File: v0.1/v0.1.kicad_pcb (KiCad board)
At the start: 4 copper layers, 66.4 x 47.2 mm, 147 parts, among them J1 Conn_01x05_Pin, J2 Conn_01x04_Pin, J3 Conn_01x02_Pin, J4 Conn_01x02_Pin, U1 XC6206P152MR, U10 STM32U5G9ZJTxQ, U2 XC6206P282MR, U3 SY8088AAC, U4 XC6206P282MR, U9 MX66LM1G45G, X1 32.768kHz, X2 16MHz

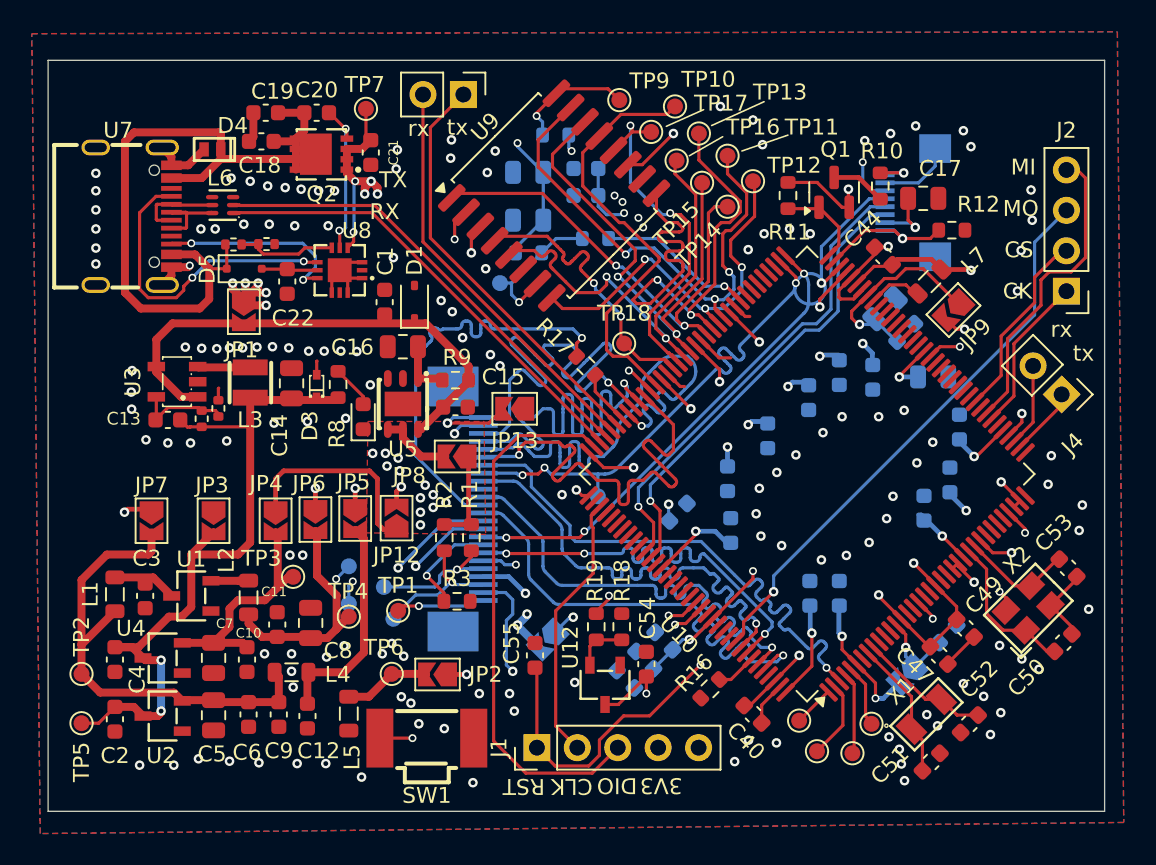
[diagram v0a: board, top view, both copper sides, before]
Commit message: [HW] [PCB] PCB Revision 0.2_Y50; DK1
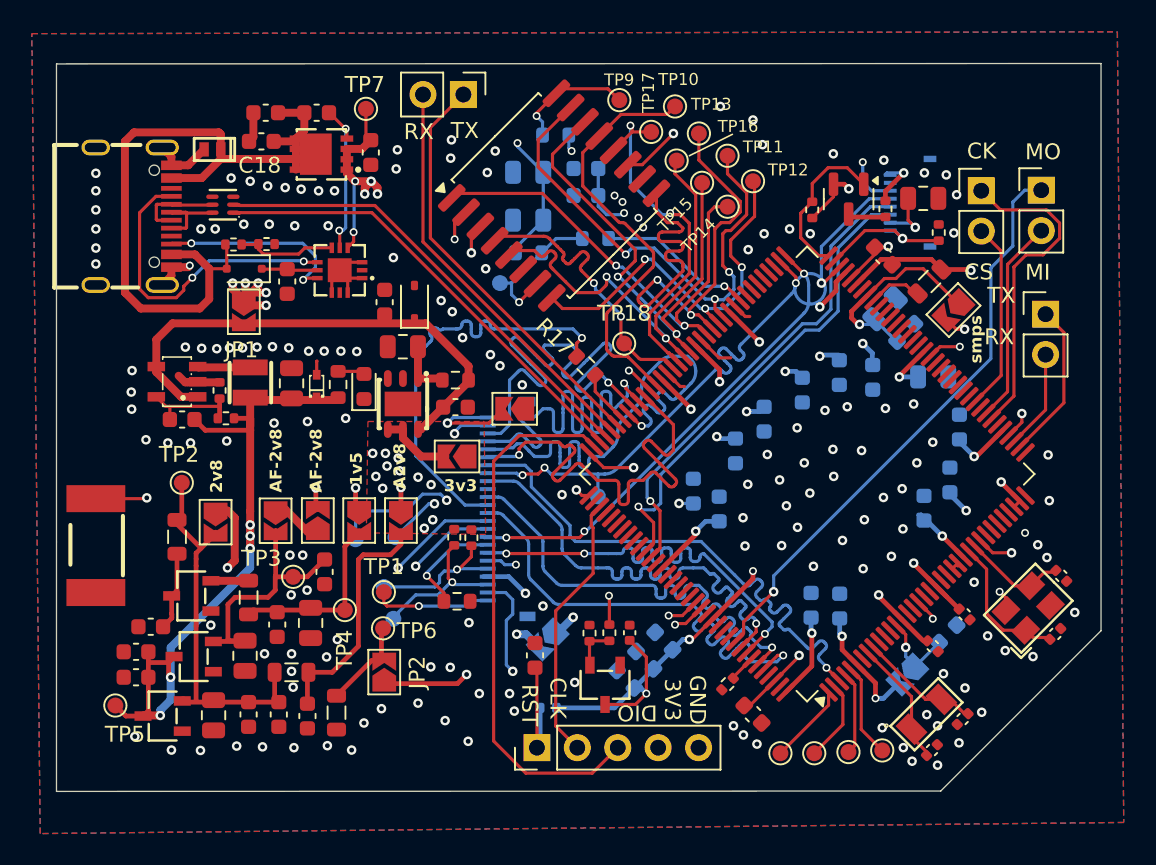
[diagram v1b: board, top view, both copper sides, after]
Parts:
- removed the JP3 at (93.9, 76.5)
- added J3: Conn_01x02_Pin, Connector_PinHeader_2.54mm:PinHeader_1x02_P2.54mm_Vertical, F.Cu at (142.2, 55.8)
- added R20: 100k, Resistor_SMD:R_0402_1005Metric, B.Cu at (114.9, 88.3)
- C47, C49, C50, C51, C52, C53, C54: footprint Capacitor_SMD:C_0603_1608Metric -> Capacitor_SMD:C_0402_1005Metric
- J2: value Conn_01x04_Pin -> Conn_01x02_Pin; footprint Connector_PinHeader_2.54mm:PinHeader_1x04_P2.54mm_Vertical -> Connector_PinHeader_2.54mm:PinHeader_1x02_P2.54mm_Vertical
- R1, R16, R18, R19, R2: footprint Resistor_SMD:R_0603_1608Metric -> Resistor_SMD:R_0402_1005Metric
- R10: renamed from R12; footprint Resistor_SMD:R_0603_1608Metric -> Resistor_SMD:R_0402_1005Metric
- R11: renamed from R10; footprint Resistor_SMD:R_0603_1608Metric -> Resistor_SMD:R_0402_1005Metric
- R12: renamed from R11; footprint Resistor_SMD:R_0603_1608Metric -> Resistor_SMD:R_0402_1005Metric
- R4, R5: value 27R -> 33R
- U11: footprint Grinreflex:FPC-SMD_24P-P0.50_SHOU-HAN_CTSJ-H2.0 -> Grinreflex:FFC-SMD_24P-P0.50_FH34SRJ-24S-0.5SH
- U6: footprint Grinreflex:FPC-SMD_8P-P0.50_AFC24-S08FCA-00 -> Grinreflex:FPC-SMD_8P-P0.50_FH34D-8S-0.5SH-50
- moved SW1 24.1 mm to (86.5, 78.1), turned to 90 degrees
- moved TP2 13.6 mm to (91.9, 74.2)
- moved C10 7.36 mm to (100.9, 79.8)
- moved J2 6.54 mm to (145.9, 55.8), turned to 0 degrees
- moved L1 5.32 mm to (91.6, 77.5), turned to -90 degrees
- moved J5 5.15 mm to (146.2, 63.6), turned to 0 degrees
- moved JP11 4.95 mm to (100.5, 76.5)
- moved TP24 4.07 mm to (102.8, 77.7)
- moved JP6 4.03 mm to (94.0, 76.6)
- moved TP23 3.45 mm to (105.3, 77.6)
- moved JP2 3.35 mm to (104.6, 86.0), turned to 90 degrees
- moved C2 2.95 mm to (89.0, 86.4), turned to 180 degrees
- moved TP6 2.91 mm to (104.5, 83.3)
- moved JP4 2.88 mm to (105.7, 76.5)
- moved JP5 2.75 mm to (103.0, 76.5)
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- renumbered J3 to J4, J4 to J5, JP11 to JP10, JP12 to JP11, JP13 to JP12, JP4 to JP3, JP5 to JP4, JP6 to JP5, JP7 to JP6, JP8 to JP7, JP9 to JP8, JP10 to JP9
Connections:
- C22 pad 1: Net-(D5-A) -> Net-(D5-K)
- D5 pad 1: /USB-C/VBUS -> Net-(D5-K)
- D5 pad 2: Net-(D5-A) -> /USB-C/VBUS
- J2 pad 1: /MCU/spi1_sck -> /MCU/spi1_mosi
- J2 pad 2: /MCU/spi1_nss -> /MCU/spi1_miso
- U10 pad 119: /LCD/LCD_SDA -> /LCD/LCD_SCL
- U10 pad 120: /LCD/LCD_SCL -> /LCD/LCD_SDA
- U8 pad 8: Net-(D5-A) -> Net-(D5-K)
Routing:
- net /RESET: track 149.4 -> 168.8 mm, vias 7 -> 6
- net GND: track 52.6 -> 33.3 mm, vias 150 -> 162
- net /MCU/spi1_sck: track 9.96 -> 20.4 mm
- net /AF-2v8: track 12.9 -> 3.25 mm
- net /MCU/spi1_miso: track 19.6 -> 12.9 mm
- net /Power/2v8: track 30.4 -> 24.2 mm
- net /MCU/usart2_tx: track 4.38 -> 9.96 mm
- net Net-(JP11-B): track 8.22 -> 13.6 mm
- net /2v8: track 27.0 -> 22.0 mm
- net /Camera/DVP_VSYNC: track 41.6 -> 37.1 mm
- net /GNDA: track 11.0 -> 15.4 mm
- net /LCD/lcd_led: track 5.81 -> 10.0 mm
- net Net-(D5-K): track 0.00 -> 3.53 mm
- net Net-(D5-A): track 3.53 -> 0.00 mm
- net /DVDD-1v5: track 16.5 -> 13.1 mm
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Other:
- board size 66.4 x 47.2 mm -> 65.7 x 45.8 mm
- board text added: "1"
- board text added: "1v5"
- board text added: "24"
- board text added: "2v8"
- board text added: "3v3"
- board text added: "8"
- board text added: "A2v8"
- board text added: "AF-2v8"
- board text added: "DSI"
- board text added: "GND"
- board text added: "GrinReflex DK1"
- board text added: "REV 0.2 15.08.2025"
- board text added: "USB"
- board text added: "smps"
- board text removed: "rx"
- board text removed: "tx"
